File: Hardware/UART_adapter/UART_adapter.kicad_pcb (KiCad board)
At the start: 2 copper layers, 99.5 x 34.5 mm, 3 parts, among them J2 Conn_02x07_Top_Bottom

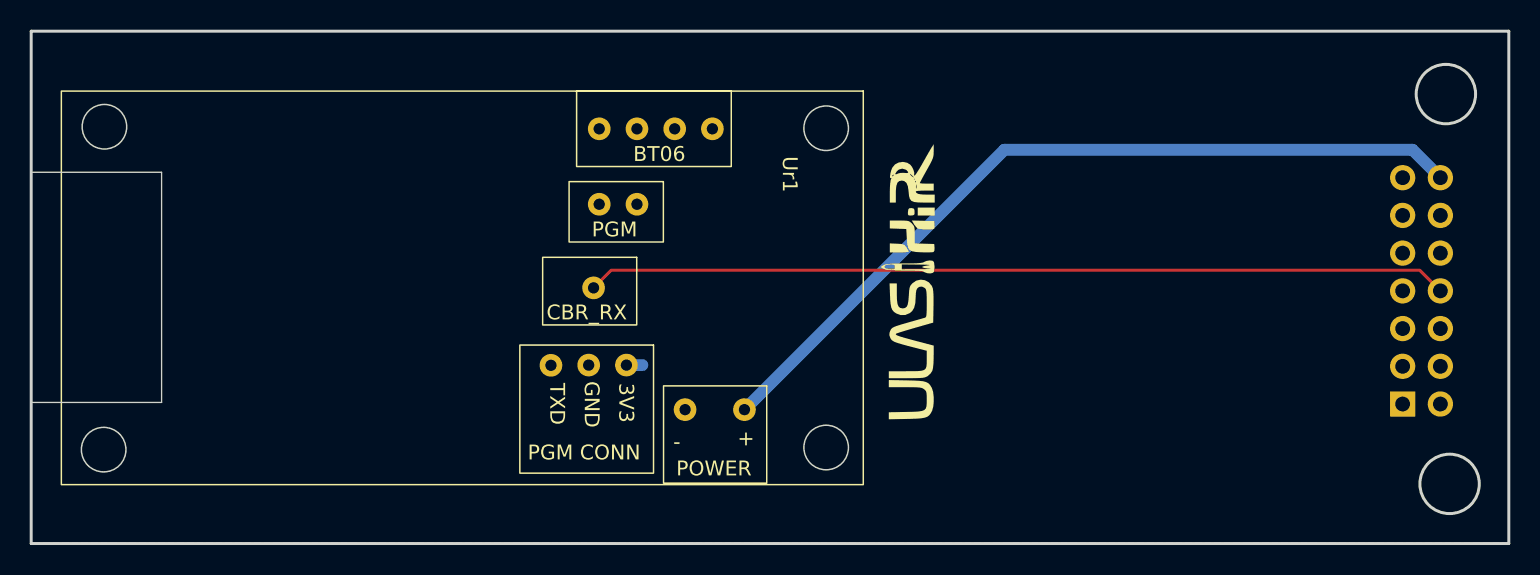
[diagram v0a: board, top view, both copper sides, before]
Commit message: hardware done
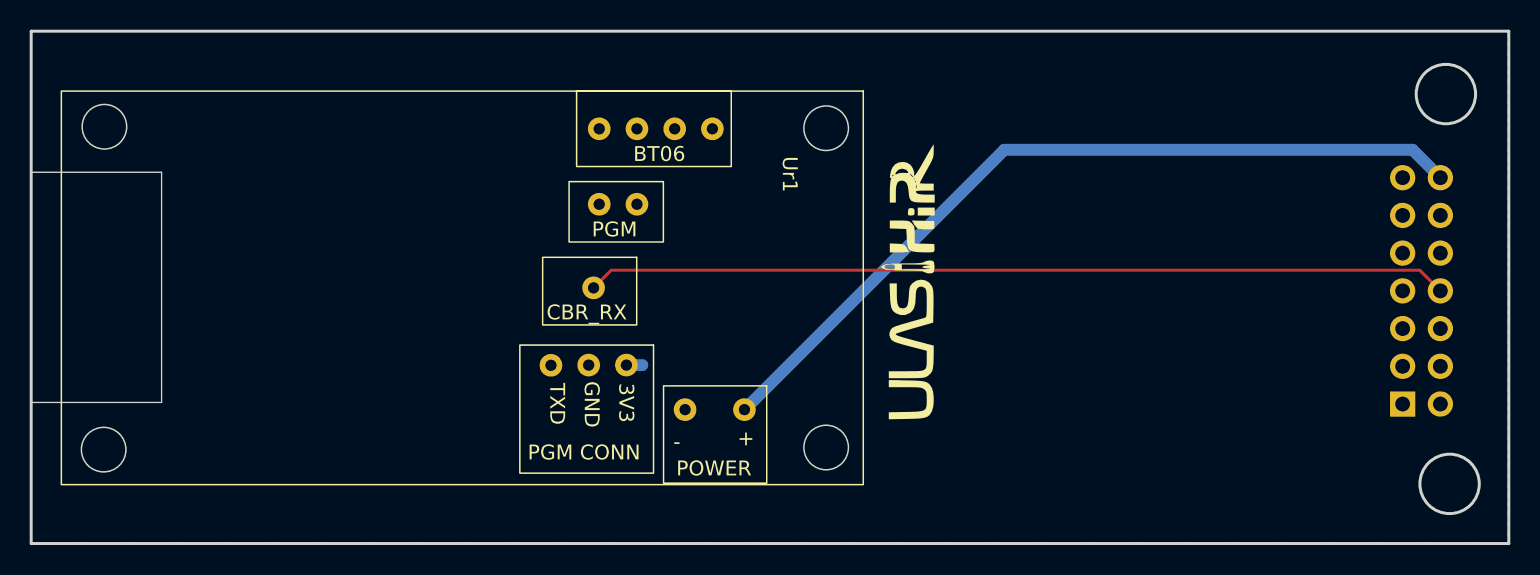
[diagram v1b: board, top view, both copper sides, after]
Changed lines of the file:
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@@
 			(drillshape 0)
 			(scaleselection 1)
-			(outputdirectory "../Manufacturing/UART_adapter/Gerber Output/")
+			(outputdirectory "../Manufacturing/UART_adapter/fabrication/")
 		)
 	)
@@
 		(net 6)
 		(net_name "GND")
-		(layer "F.Cu")
+		(layers "F.Cu" "B.Cu")
 		(hatch edge 0.5)
 		(priority 1)
